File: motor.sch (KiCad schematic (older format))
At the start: 44 parts, among them J16 70543-0003, Q10 PMPB20EN, Q3 PMPB20EN, Q4 PMPB20EN, Q5 PMPB20EN, Q6 PMPB20EN, Q7 PMPB20EN, Q8 PMPB20EN, Q9 PMPB20EN, U6 TMC2160-TA

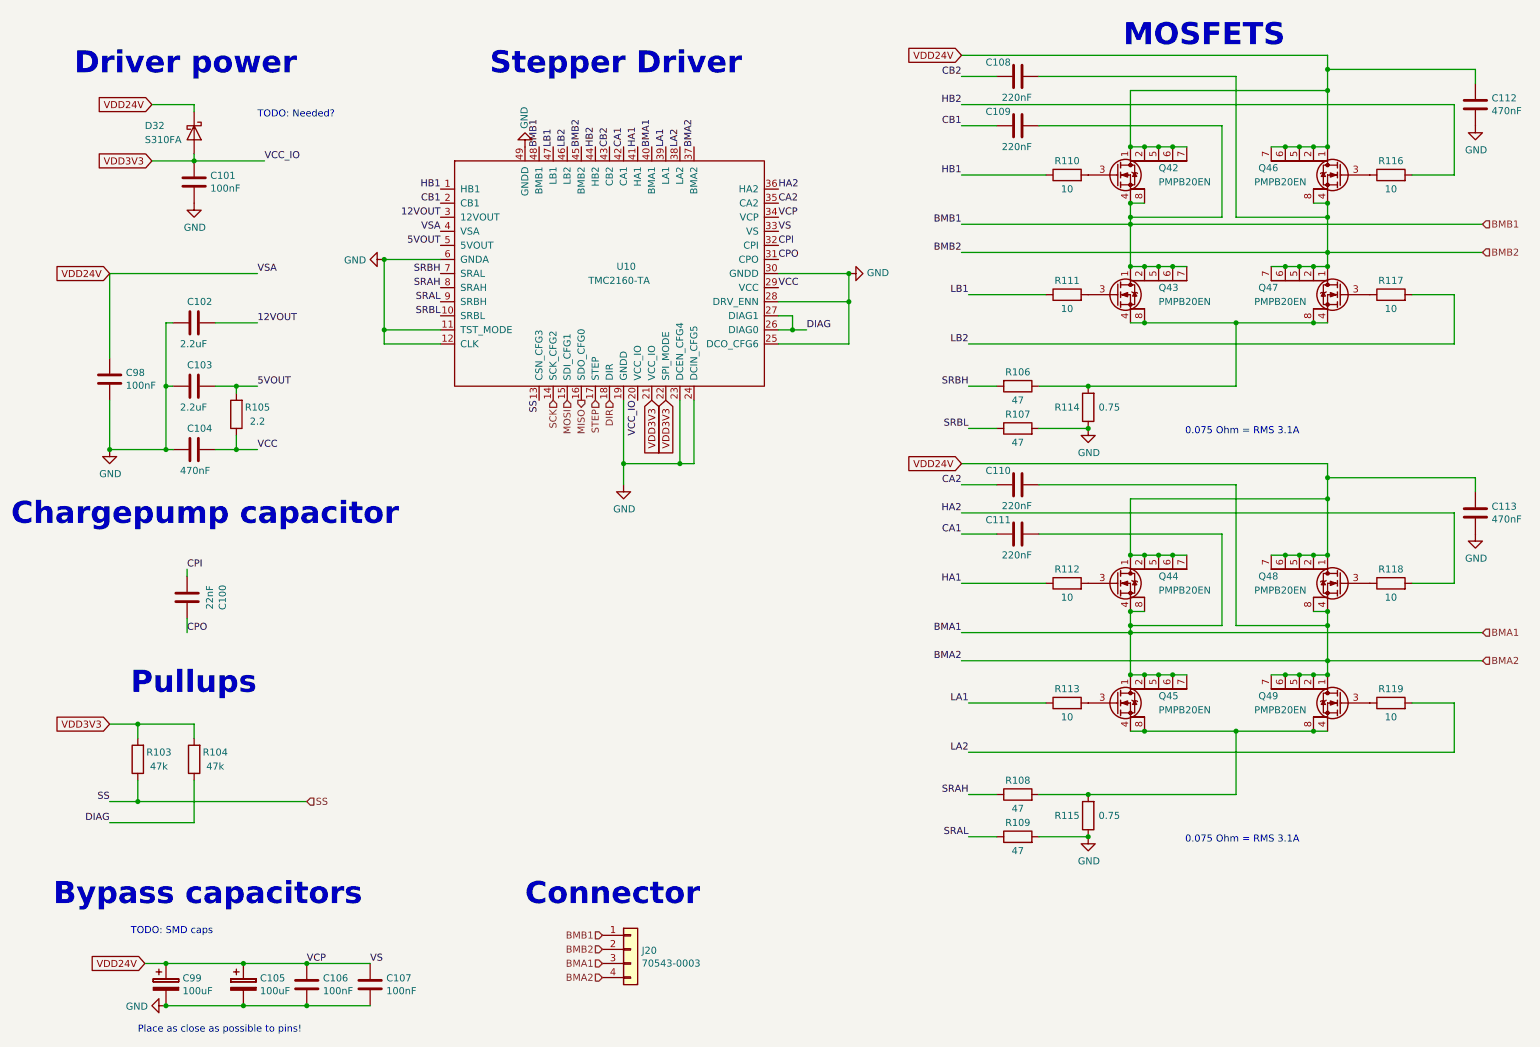
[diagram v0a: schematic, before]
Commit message: First pass of routing
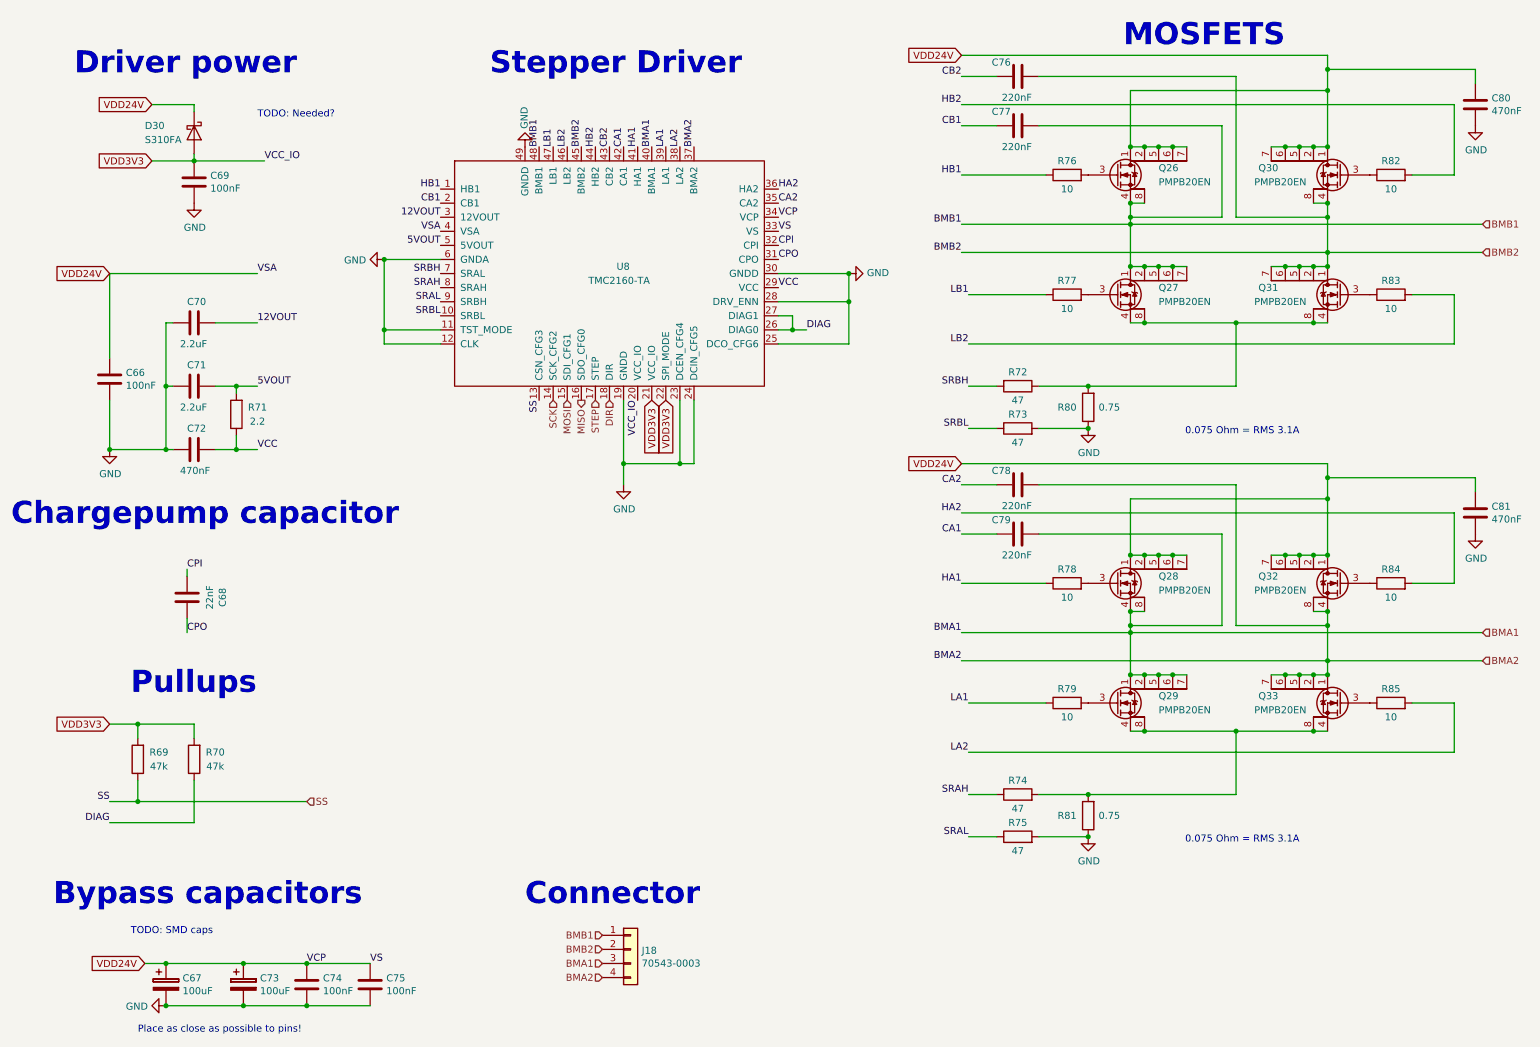
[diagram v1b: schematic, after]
